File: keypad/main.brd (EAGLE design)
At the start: 160 x 100 mm, 23 parts

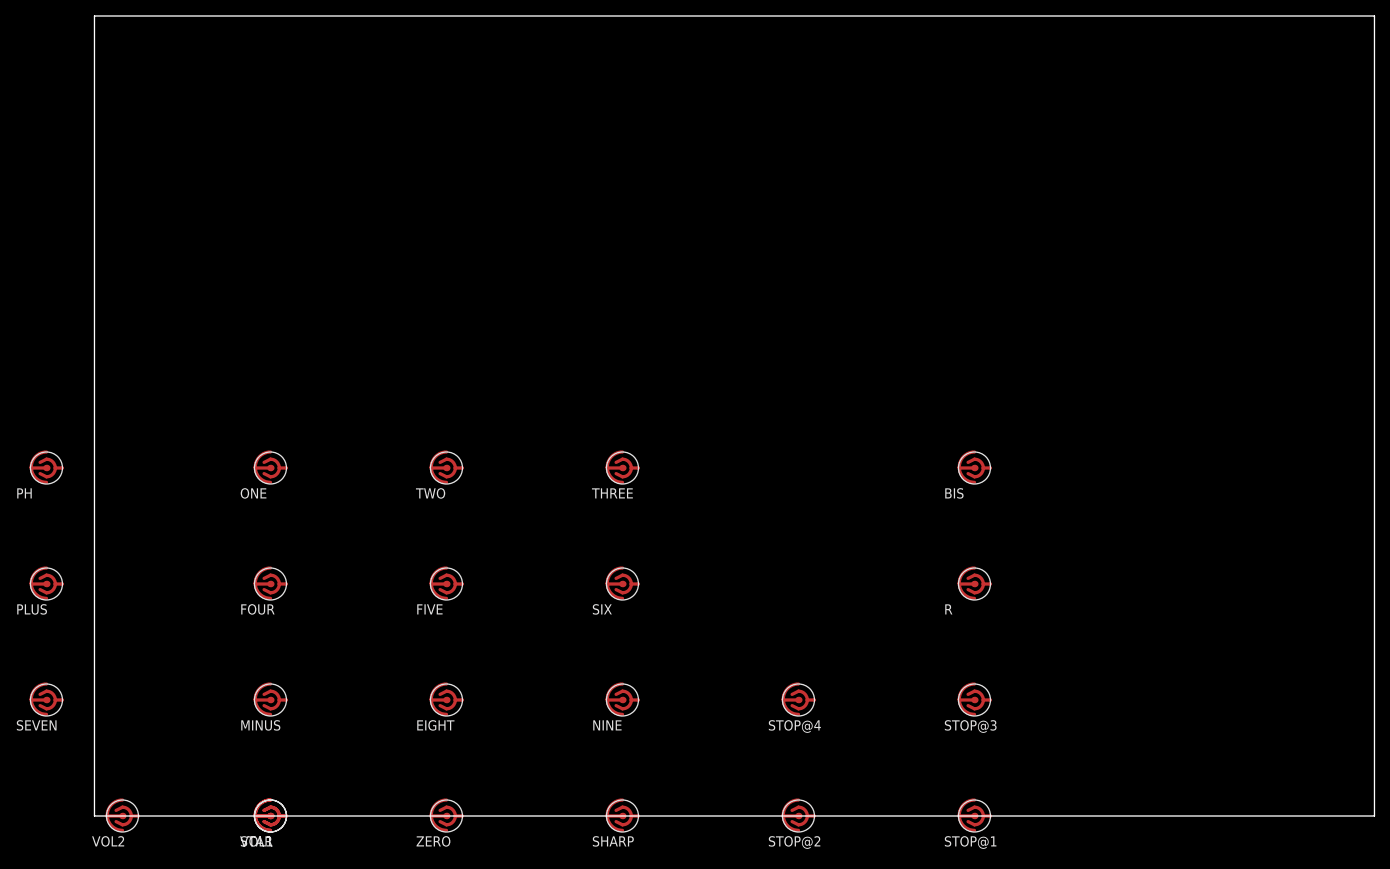
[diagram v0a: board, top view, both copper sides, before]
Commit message: updated project
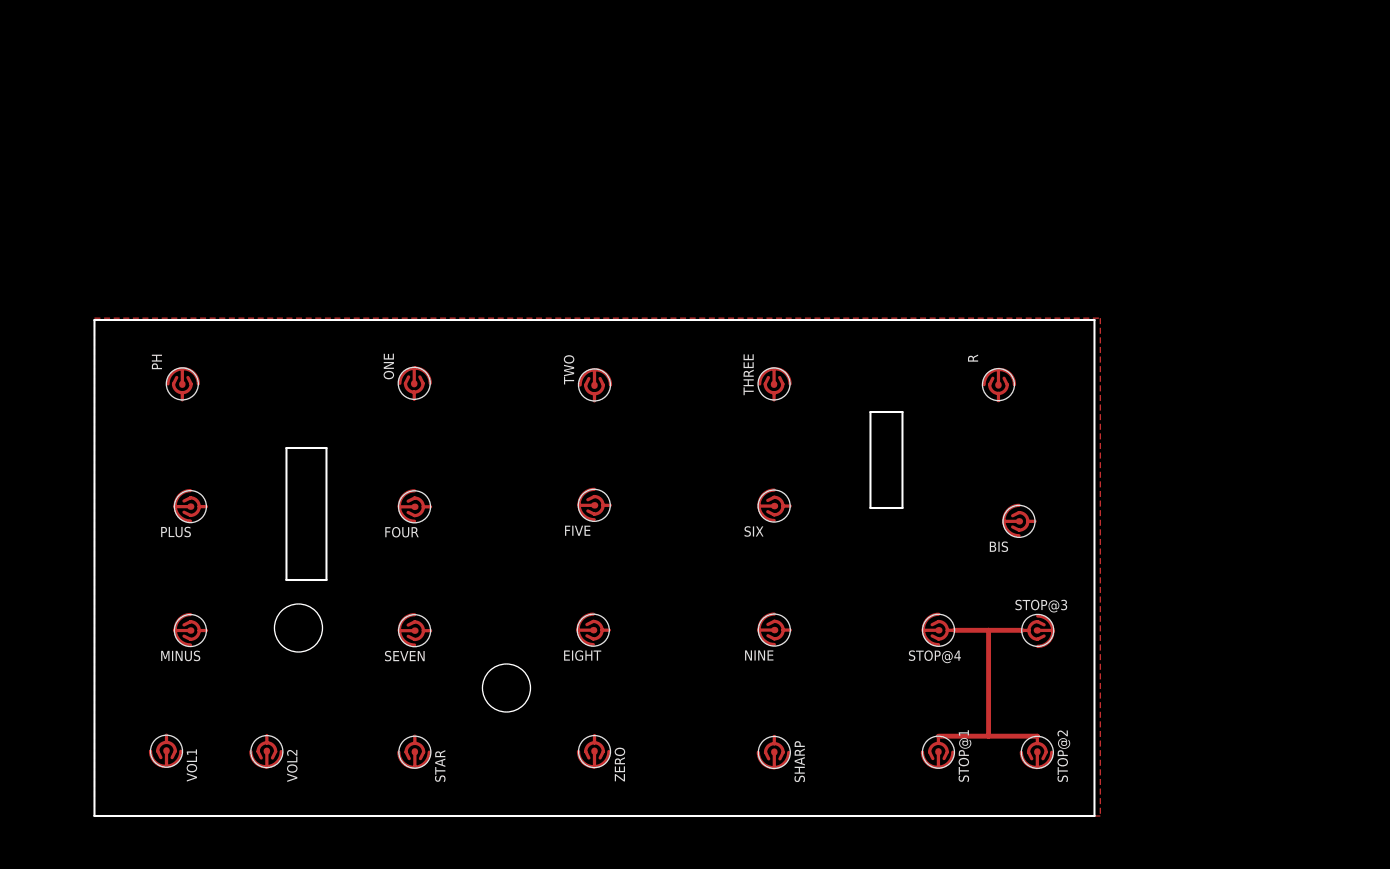
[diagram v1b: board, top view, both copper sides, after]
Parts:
- moved SEVEN 46.8 mm to (40.0, 23.2)
- moved STOP@2 30.9 mm to (117.9, 7.96), turned to 90 degrees
- moved R 25.1 mm to (113.0, 53.9), turned to 270 degrees
- moved THREE 21.7 mm to (84.9, 54.0), turned to 270 degrees
- moved SIX 21.3 mm to (85.0, 38.7)
- moved TWO 21.2 mm to (62.5, 53.9), turned to 270 degrees
- moved FIVE 20.9 mm to (62.5, 38.8)
- moved NINE 20.9 mm to (85.0, 23.2)
- moved ONE 20.9 mm to (40.0, 54.1), turned to 270 degrees
- moved SHARP 20.6 mm to (85.0, 7.94), turned to 90 degrees
- moved FOUR 20.4 mm to (40.0, 38.6)
- moved PLUS 20.4 mm to (12.0, 38.7)
- moved EIGHT 20.3 mm to (62.4, 23.2)
- moved ZERO 20.2 mm to (62.5, 8.05), turned to 90 degrees
- moved PH 20.0 mm to (11.0, 54.0), turned to 270 degrees
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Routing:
- net N$2: track 0.00 -> 34.0 mm
- added copper zone on layer 1, net GND
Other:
- board size 160 x 100 mm -> 125 x 62 mm
